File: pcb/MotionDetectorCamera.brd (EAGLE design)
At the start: 64.8 x 50.8 mm, 129 parts, among them J2 S-MOUNT-LENS-HOLDER, U1 LATTICE-ICE40HX4K-BG121, U10 NXP-NTB0102, U11 ON-NLAS3157, U12 ON-NLAS3157, U13 STM-STM32F730, U2 TI-TPS6280XYKAR, U3 MICROSD-SOCKET, U4 TI-TPS6280XYKAR, U5 W989D6DBGX6I, U6 TI-TPS63805YFFR, U8 ON-AR0330CS1C12SPKA0, U9 TI-TMUX1574, X1 SITIME-SIT8021, X2 SITIME-SIT8021

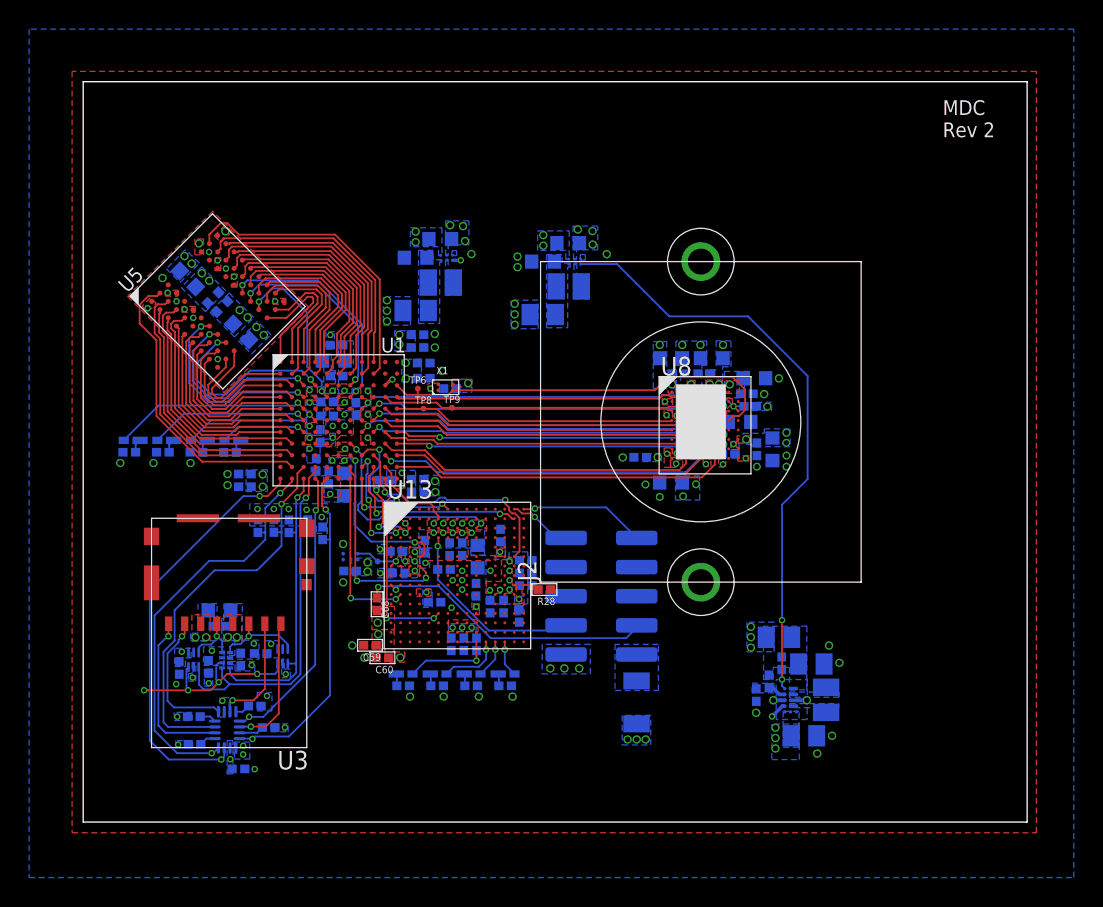
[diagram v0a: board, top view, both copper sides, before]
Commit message: Layout progress
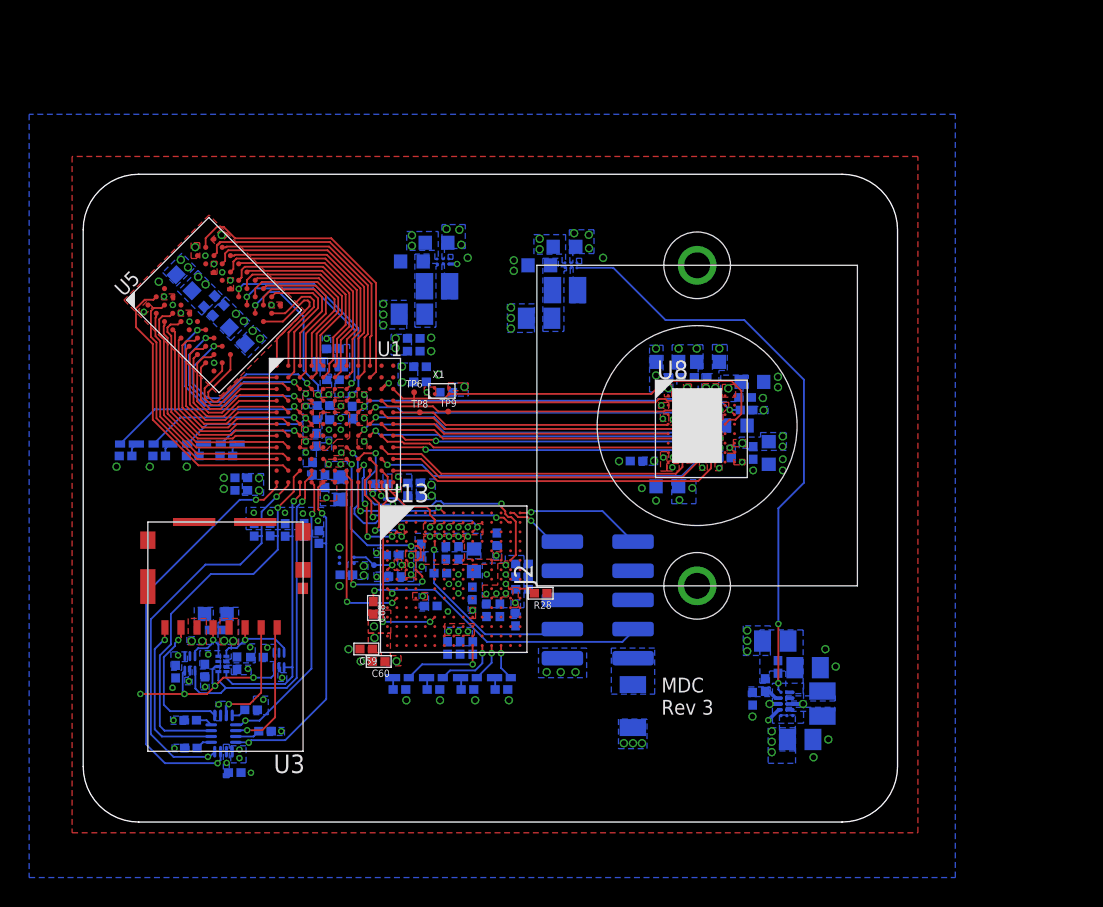
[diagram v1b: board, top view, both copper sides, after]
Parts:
- moved C18 0.36 mm to (22.6, 38.5)
- moved C37 0.36 mm to (47.0, 25.3)
- moved C39 0.36 mm to (42.4, 30.5)
- moved C41 0.36 mm to (38.0, 24.8)
- moved C43 0.36 mm to (46.0, 25.3)
- moved L4 0.36 mm to (24.3, 36.8)
- moved R12 0.36 mm to (31.3, 34.6)
- moved R6 0.36 mm to (22.6, 34.8)
- moved C26 0.36 mm to (10.6, 33.4)
- moved H1 0.36 mm to (35.3, 15.2)
- moved L2 0.36 mm to (50.7, 8.13)
- moved R18 0.36 mm to (46.8, 9.40)
- moved C13 0.36 mm to (16.5, 28.6)
- moved C15 0.36 mm to (16.5, 27.6)
- moved C17 0.36 mm to (16.0, 26.2)
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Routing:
- net GND: vias 96 -> 97
- net 2V8: vias 26 -> 27
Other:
- board size 64.8 x 50.8 mm -> 55.9 x 44.5 mm
- board text added: "MDC Rev 3"
- board text removed: "MDC Rev 2"
